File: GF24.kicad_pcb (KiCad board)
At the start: 4 copper layers, 82 x 40 mm, 69 parts, among them J1 USB4110GFA, J2 S2B-PH-SM4-TB, J3 Conn_01x06_Pin, J4 Conn_01x06_Pin, J5 Conn_ARM_SWD_TagConnect_TC2030, J6 Conn_01x04_Pin, Q1 3904, SW4 BOOT, SW5 1-1825027-7, U1 TPS79533DCQR, U2 LTC1733, U3 SAM-M10Q, U4 STM32F102C8Tx, X1 ECS-2520MV-160-CN

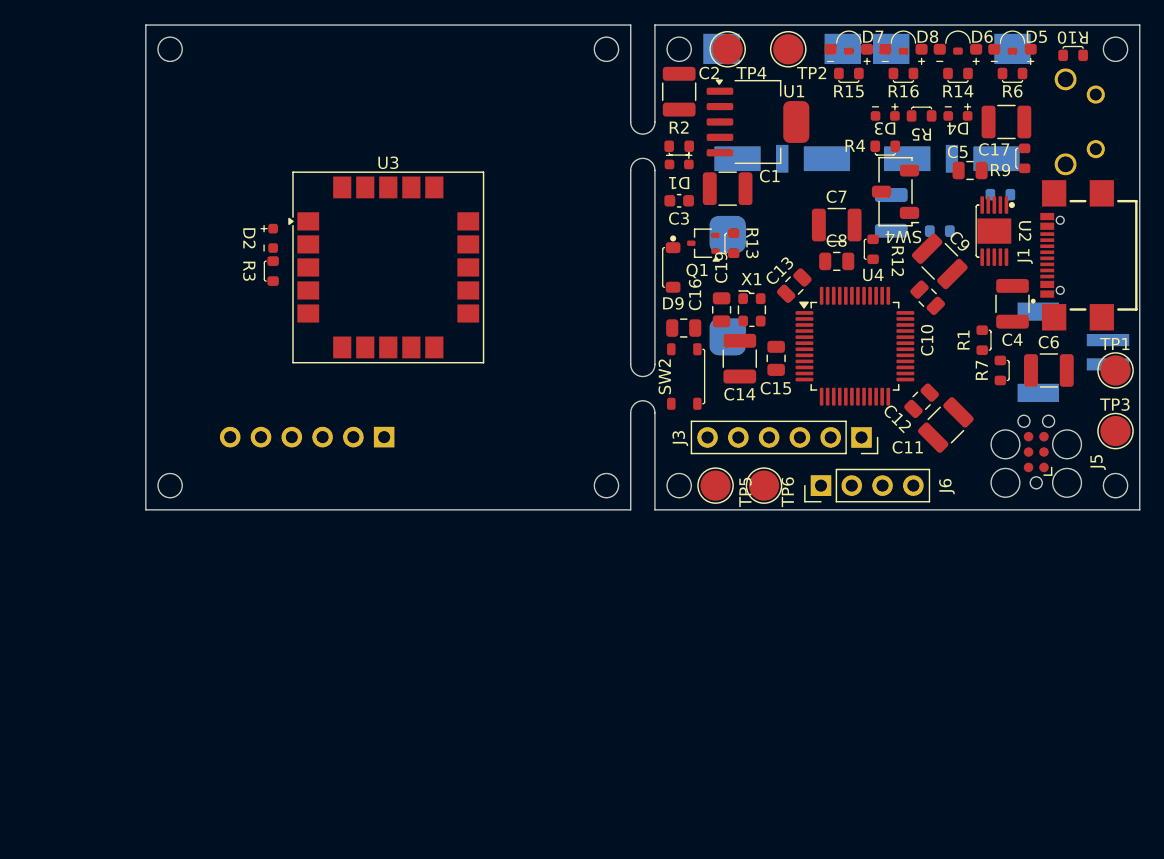
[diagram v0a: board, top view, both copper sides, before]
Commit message: 3D done, started routing
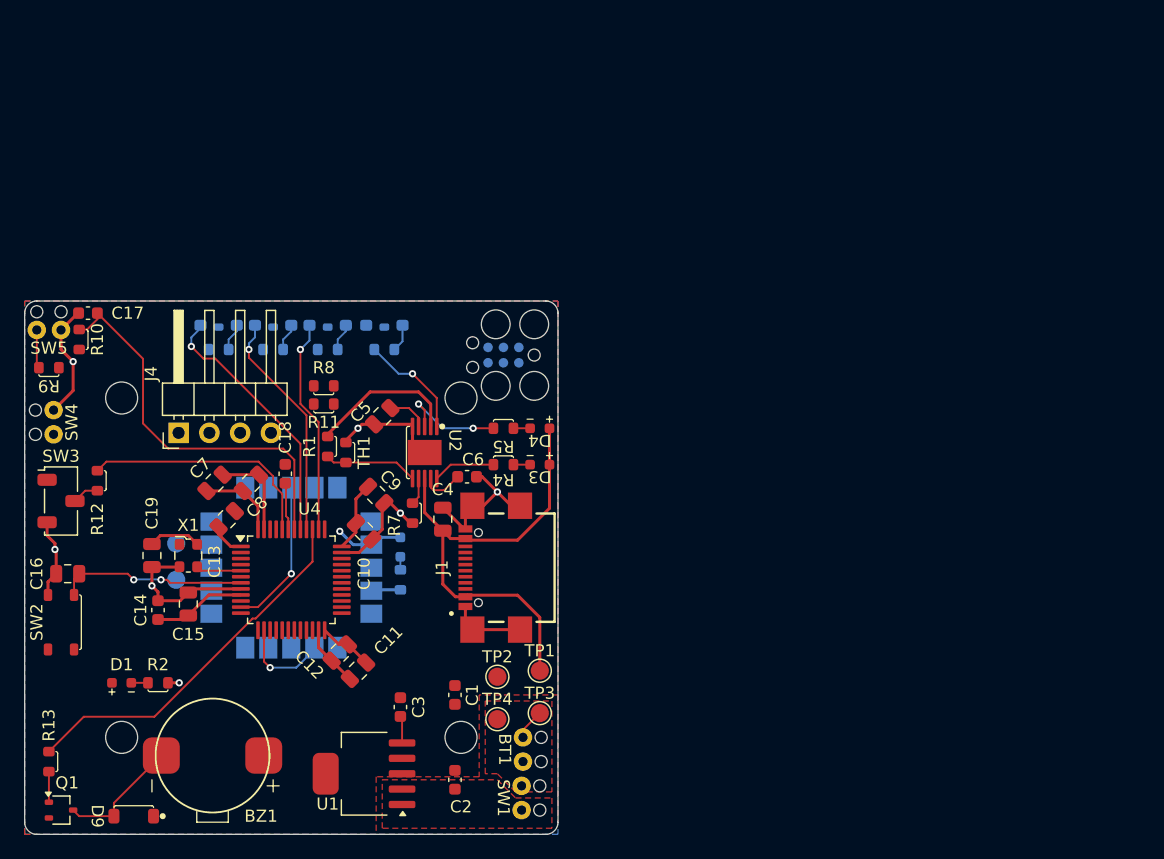
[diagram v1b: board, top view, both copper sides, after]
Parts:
- removed J2: S2B-PH-SM4-TB, MB-Conn:JST_S2B-PH-SM4-TB
- removed J5: Conn_ARM_SWD_TagConnect_TC2030, Connector:Tag-Connect_TC2030-IDC-FP_2x03_P1.27mm_Vertical
- removed J6: Conn_01x04_Pin, Connector_PinHeader_2.54mm:PinHeader_1x04_P2.54mm_Vertical
- added BT1: Battery_Cell, MB-SW:Solder_Joint_1_2, F.Cu at (89.1, 87.0)
- BZ1, R11, R8, TH1: moved to F.Cu
- C1, C14, C17, C2, C6: footprint Capacitor_SMD:C_1210_3225Metric -> Capacitor_SMD:C_0603_1608Metric
- C11, C4, C7, C9: footprint Capacitor_SMD:C_1210_3225Metric -> Capacitor_SMD:C_0805_2012Metric
- C18: footprint Capacitor_SMD:C_1210_3225Metric -> Capacitor_SMD:C_0603_1608Metric; moved to F.Cu
- D2, D5, D6, D7, D8, R14, R15, R16, R3, R6, U3: moved to B.Cu
- J3: value Conn_01x06_Pin -> Conn_ARM_SWD_TagConnect_TC2030; footprint Connector_PinSocket_2.54mm:PinSocket_1x06_P2.54mm_Vertical -> Connector:Tag-Connect_TC2030-IDC-FP_2x03_P1.27mm_Vertical; moved to B.Cu
- J4: value Conn_01x06_Pin -> Conn_01x04_Pin; footprint Connector_PinHeader_2.54mm:PinHeader_1x06_P2.54mm_Vertical -> Connector_PinHeader_2.54mm:PinHeader_1x04_P2.54mm_Horizontal; moved to F.Cu
- SW1: value ~ -> EG1205; footprint MB-SW:SW_500ASSP1SM6QE -> MB-SW:Solder_Joint_1_2; moved to F.Cu
- SW3: value ~ -> BOOT; footprint MB-SW:SW_500ASSP1SM6QE -> Button_Switch_SMD:Nidec_Copal_CAS-120A; moved to F.Cu
- SW4: value BOOT -> EG1205; footprint Button_Switch_SMD:Nidec_Copal_CAS-120A -> MB-SW:Solder_Joint_1_2
- SW5: value 1-1825027-7 -> 360-2674-ND; footprint MB-SW:SW2_1825027-F_TEC -> MB-SW:Solder_Joint_1_2; moved to F.Cu
- TP1, TP2, TP3, TP4: footprint TestPoint:TestPoint_Pad_D2.5mm -> TestPoint:TestPoint_Pad_D1.5mm
- TP5, TP6: footprint TestPoint:TestPoint_Pad_D2.5mm -> TestPoint:TestPoint_Pad_D1.5mm; moved to B.Cu
- moved SW5 89.0 mm to (52.0, 54.4), turned to 0 degrees
- moved R10 85.3 mm to (54.5, 53.2), turned to 90 degrees
- moved R9 82.3 mm to (52.0, 55.5), turned to 0 degrees
- moved SW3 80.5 mm to (53.0, 66.5)
- moved C17 77.4 mm to (55.2, 51.0)
- moved R13 70.9 mm to (52.0, 88.0), turned to 90 degrees
- moved Q1 70.7 mm to (53.0, 92.0), turned to 0 degrees
- moved SW4 70.1 mm to (54.4, 60.0), turned to 90 degrees
- moved R12 66.8 mm to (56.0, 64.8), turned to 90 degrees
- moved D9 63.5 mm to (59.0, 92.5), turned to 180 degrees
- moved U1 62.8 mm to (78.0, 89.0), turned to 180 degrees
- moved D1 62.8 mm to (58.0, 81.5), turned to 0 degrees
- moved SW1 61.9 mm to (89.0, 91.0), turned to -90 degrees
- moved R2 61.7 mm to (61.0, 81.5)
- moved C2 59.7 mm to (85.5, 89.5)
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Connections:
- net Net-(D3-A) renamed /USBC+
- net Net-(U1-NR) renamed /Noise_Reduction
- net Net-(U4-BOOT0) renamed /BOOT0_I
- net Net-(U4-PD0) renamed /CLK_OUT
- C6 pad 1: Net-(U2-BAT) -> BAT+
- D2 pad 2: GNSS-3V3 -> +3V3
- J3 pad 1: GND -> +3V3
- J3 pad 2: /GNSS-ST-TIMEPULSE -> /SWDIO
- J3 pad 3: /GNSS-ST-RX2 -> NRST
- J3 pad 4: /GNSS-ST-TX2 -> /SWDCLK
- J3 pad 5: /GNSS-ST-N-RESET -> GND
- J3 pad 6: +3V3 -> unconnected-(J3-SWO-Pad6)
- J4 pad 1: GNSS-GND -> +3V3
- J4 pad 2: GNSS-TIMEPULSE -> /DEBUG_ST_TX
- J4 pad 3: GNSS-TX -> /DEBUG_ST_RX
- J4 pad 4: GNSS-RX -> GND
- R3 pad 2: GNSS-GND -> GND
- SW3 pad 1: /MODE-H -> +3V3
- SW3 pad 2: GND -> /BOOT0_RES
- SW3 pad 3: unconnected-(SW3-Pad3) -> GND
- SW4 pad 1: +3V3 -> /MODE-H
- SW4 pad 2: /BOOT0_RES -> GND
- TP3 pad 1: Net-(U2-BAT) -> BAT+
- TP5 pad 1: /GNSS-ST-TX2 -> GNSS-RX
- TP6 pad 1: /GNSS-ST-RX2 -> GNSS-TX
- U2 pad 9: Net-(U2-BAT) -> BAT+
- U3 pad 1: GNSS-GND -> GND
- U3 pad 10: GNSS-GND -> GND
- U3 pad 11: GNSS-GND -> GND
- U3 pad 15: GNSS-GND -> GND
- U3 pad 16: GNSS-GND -> GND
- U3 pad 17: GNSS-3V3 -> +3V3
- U3 pad 2: GNSS-3V3 -> +3V3
- U3 pad 20: GNSS-GND -> GND
- U3 pad 4: GNSS-GND -> GND
- U3 pad 5: GNSS-GND -> GND
- U3 pad 6: GNSS-GND -> GND
- U4 pad 11: /GNSS-ST-N-RESET -> GNSS-N-RESET
- U4 pad 12: /GNSS-ST-TX2 -> GNSS-RX
- U4 pad 13: /GNSS-ST-RX2 -> GNSS-TX
- U4 pad 14: /GNSS-ST-TIMEPULSE -> GNSS-TIMEPULSE
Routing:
- net GND: track 0.00 -> 81.2 mm, vias 0 -> 7
- net /USBC+: track 0.00 -> 52.3 mm
- net +3V3: track 0.00 -> 37.6 mm, vias 0 -> 1
- net BUTTON: track 0.00 -> 32.5 mm
- net BUZZER: track 0.00 -> 30.9 mm
- net STATG: track 0.00 -> 21.4 mm, vias 0 -> 1
- net /BOOT0_I: track 0.00 -> 20.0 mm
- net STATR: track 0.00 -> 19.0 mm, vias 0 -> 1
- net STATGPS: track 0.00 -> 17.8 mm, vias 0 -> 1
- net NRST: track 0.00 -> 15.6 mm, vias 0 -> 2
- net GNSS-N-RESET: track 0.00 -> 12.4 mm, vias 0 -> 1
- net /BUZZ-: track 0.00 -> 10.2 mm
- net NCHRG: track 0.00 -> 9.16 mm, vias 0 -> 1
- net NFAULT: track 0.00 -> 9.06 mm, vias 0 -> 2
- net /CH-TH-DIV: track 0.00 -> 7.76 mm
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- added copper zone on F.Cu, net +3V3
- added copper zone on F.Cu, net /REG_I
- added copper zone on F.Cu, net BAT+
- added copper zone on B.Cu, net GND
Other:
- board size 82 x 40 mm -> 44 x 44 mm
- board text added: "3 degree taper 17mm lid height 0.89093mm loss per side: should be close to 43mm^2 footprint near very top but model says more than 44"
- board text added: "BATTERY H:7.1mm"
- board text added: "Mounting Point Height: 5mm Battery Height: 7.1mm Should need at least 2.5mm standoffs"
